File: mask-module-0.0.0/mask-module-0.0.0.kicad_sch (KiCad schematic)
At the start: 9 parts, among them J1 Conn_01x02, J2 USB_C_Receptacle_USB2.0, J3 Conn_01x13, J4 Conn_01x13, U1 BQ24075RGT, U2 BMD-340, U3 MCP1703Ax-330xxTT

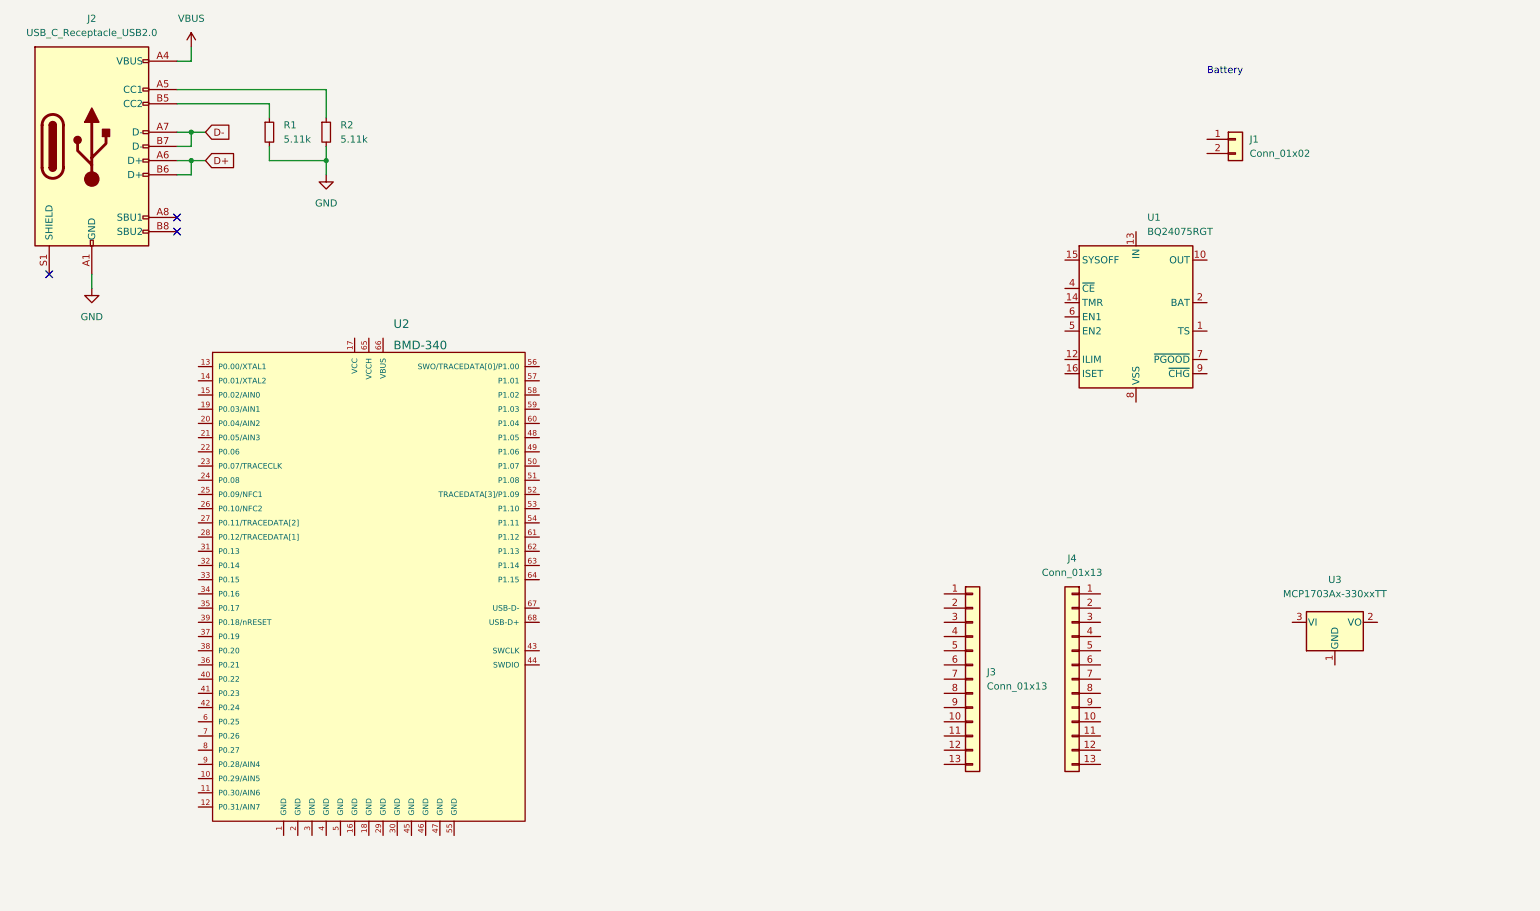
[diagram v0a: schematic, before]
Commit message: mask-module-0.0.0: update schematic
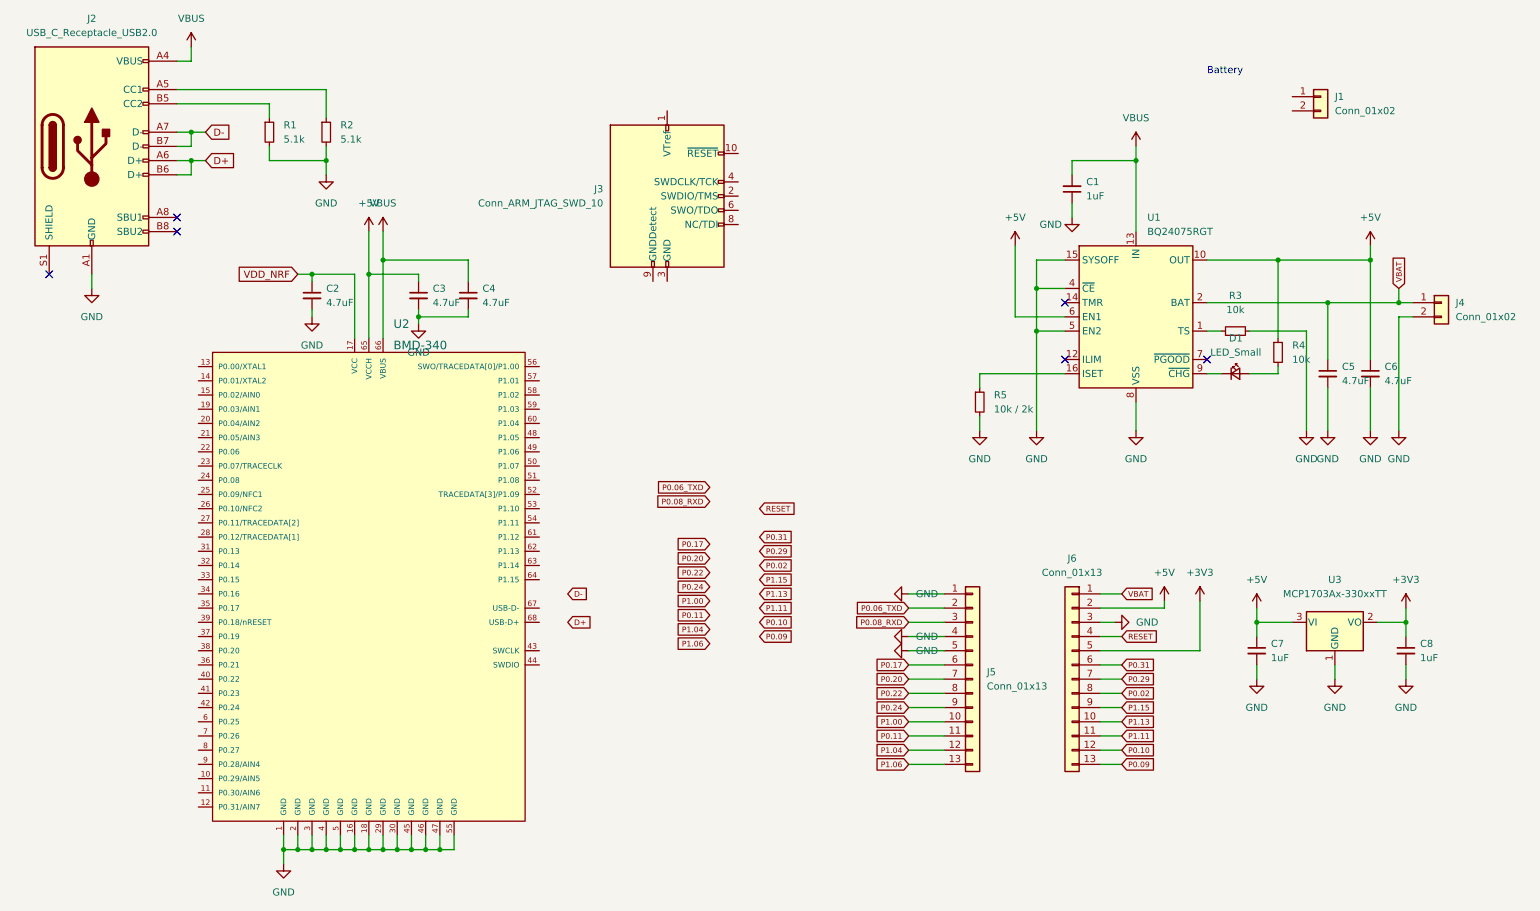
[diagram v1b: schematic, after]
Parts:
- added C1, C7, C8: 1uF, Capacitor_SMD:C_0402_1005Metric, symbol Device:C_Small
- added C2, C3, C4, C5, C6: 4.7uF, Capacitor_SMD:C_0603_1608Metric, symbol Device:C_Small
- added D1: LED_Small, LED_SMD:LED_0402_1005Metric, symbol Device:LED_Small
- added J3: Conn_ARM_JTAG_SWD_10, Connector:Tag-Connect_TC2050-IDC-NL_2x05_P1.27mm_Vertical, symbol Connector:Conn_ARM_JTAG_SWD_10
- added J4: Conn_01x02, Connector_Molex:Molex_PicoBlade_53261-0271_1x02-1MP_P1.25mm_Horizontal, symbol Connector_Generic:Conn_01x02
- added R3, R4: 10k, Resistor_SMD:R_0402_1005Metric, symbol Device:R_Small
- added R5: 10k / 2k, Resistor_SMD:R_0402_1005Metric, symbol Device:R_Small
- J2: footprint Connector_USB:USB_C_Receptacle_JAE_DX07S016JA1R1500 -> mask:USB_C_Receptacle_GCT_USB4520-xx-x-A_16P_Horizontal
- R1, R2: value 5.11k -> 5.1k; footprint Resistor_SMD:R_0603_1608Metric -> Resistor_SMD:R_0402_1005Metric
- renumbered J3 to J5, J4 to J6
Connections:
- net GND: now also J5.1 (Pin_1), J5.4 (Pin_4), J5.5 (Pin_5), J6.3 (Pin_3), U1.15 (SYSOFF), U1.17 (VSS), U1.4 (~{CE}), U1.5 (EN2), U1.8 (VSS), U2.1 (GND), U2.16 (GND), U2.18 (GND), U2.2 (GND), U2.29 (GND), U2.3 (GND), U2.30 (GND), U2.4 (GND), U2.45 (GND), U2.46 (GND), U2.47 (GND), U2.5 (GND), U2.55 (GND), U3.1 (GND), C1.1, C2.2, C3.2, C4.2, C5.2, C6.2, C7.2, C8.2, J4.2 (Pin_2), R3.2, R5.2
- net VBUS: now also U1.13 (IN), U2.66 (VBUS), C1.2, C4.1
- net P1.00: now reaches J5.10 (Pin_10)
- net P0.11: now reaches J5.11 (Pin_11)
- net P1.04: now reaches J5.12 (Pin_12)
- net P1.06: now reaches J5.13 (Pin_13)
- net P0.06_TXD: now reaches J5.2 (Pin_2)
- net P0.08_RXD: now reaches J5.3 (Pin_3)
- net P0.17: now reaches J5.6 (Pin_6)
- net P0.20: now reaches J5.7 (Pin_7)
- net P0.22: now reaches J5.8 (Pin_8)
- net P0.24: now reaches J5.9 (Pin_9)
- net VDD_NRF: now reaches U2.17 (VCC)
- net VDD_NRF: now also C2.1
- net +5V: now reaches U2.65 (VCCH)
- net +5V: now also J6.2 (Pin_2), U1.10 (OUT), U1.11 (OUT), U1.6 (EN1), U3.3 (VI), C3.1, C6.1, C7.1, R4.1
- net +3V3: now reaches U3.2 (VO)
- net +3V3: now also J6.5 (Pin_5), C8.1
- net at U1.1 (TS): now also R3.1
- net at U1.16 (ISET): now also R5.1
- net VBAT: now reaches U1.2 (BAT), U1.3 (BAT)
- net VBAT: now also J6.1 (Pin_1), C5.1, J4.1 (Pin_1)
- net at U1.9 (~{CHG}): now also D1.1 (K)
- net P1.13: now reaches J6.10 (Pin_10)
- net P1.11: now reaches J6.11 (Pin_11)
- net P0.10: now reaches J6.12 (Pin_12)
- net P0.09: now reaches J6.13 (Pin_13)
- net RESET: now reaches J6.4 (Pin_4)
- net P0.31: now reaches J6.6 (Pin_6)
- net P0.29: now reaches J6.7 (Pin_7)
- net P0.02: now reaches J6.8 (Pin_8)
- net P1.15: now reaches J6.9 (Pin_9)
- new net: D1.2 (A), R4.2
- new net: J3.3 (GND), J3.5 (GND)
- no-connect marks 3 -> 6
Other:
- moved on the sheet: J1
